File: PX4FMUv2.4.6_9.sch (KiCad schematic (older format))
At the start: 25 parts, among them J901 HEADER-3X163X16RA, U901 TXS0108QFN20, U902 TXS0108QFN20

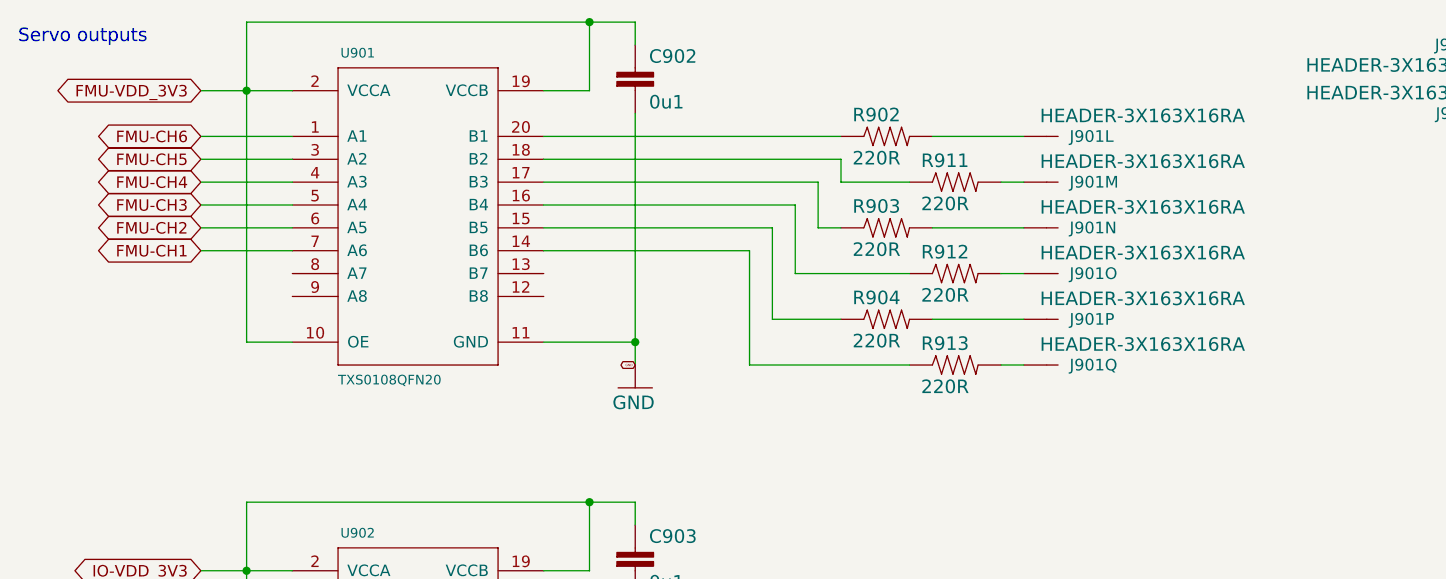
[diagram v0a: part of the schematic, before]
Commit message: removed more things
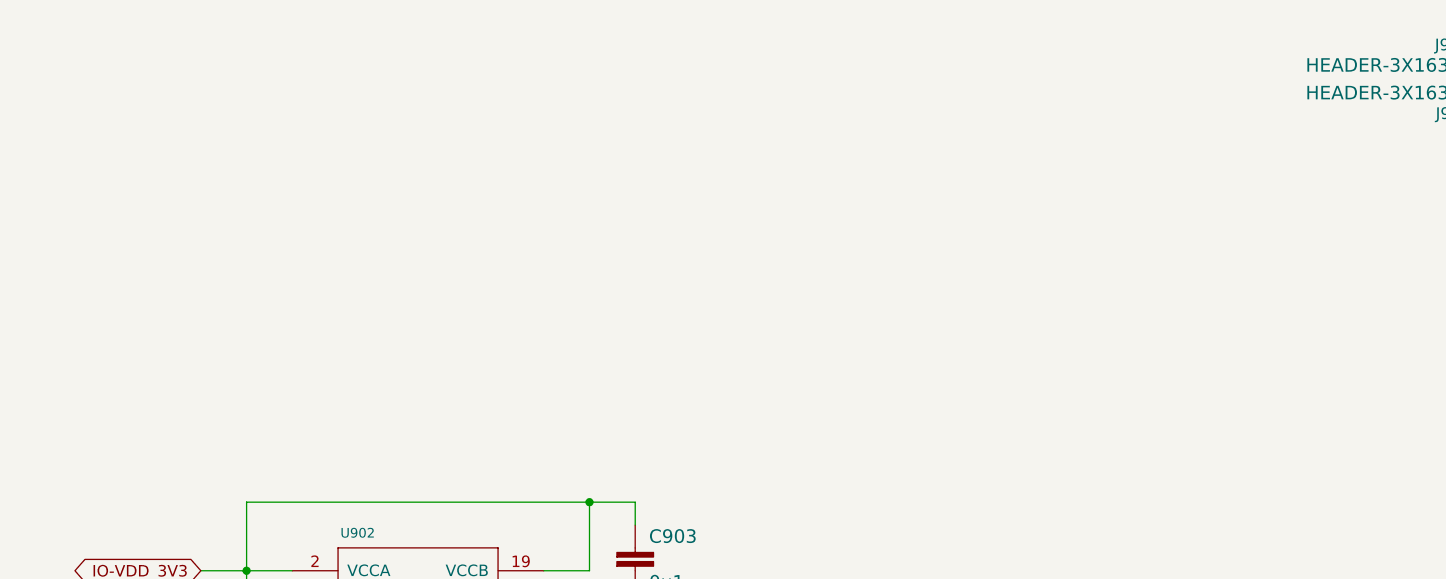
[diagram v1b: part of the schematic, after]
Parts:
- removed C902: 0u1, PX4FMUv2.4.6:0402-CAP, symbol PX4FMUv2.4.6-eagle-import:CAP0402
- removed unit 14 of J901
- removed unit 15 of J901
- removed unit 12 of J901
- removed unit 13 of J901
- removed unit 16 of J901
- removed unit 17 of J901
- removed R902, R903, R904, R911, R912, R913: 220R, PX4FMUv2.4.6:0402-RES, symbol PX4FMUv2.4.6-eagle-import:RESISTOR0402-RES
- removed U901: TXS0108QFN20, PX4FMUv2.4.6:QFN20-RGY, symbol PX4FMUv2.4.6-eagle-import:TXS0108QFN20
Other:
- note removed: "Servo outputs"
